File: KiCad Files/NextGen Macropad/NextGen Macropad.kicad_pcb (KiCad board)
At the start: 2 copper layers, 80.4 x 119.4 mm, 80 parts, among them J1 OLED_128x64, J2 Battery JST-PH, J3 USB_C_Receptacle_USB2.0_16P, Q1 AO3401A, SW1 SW_Push_45deg, SW10 SW_Push_45deg, SW11 SW_Push_45deg, SW12 SW_Push_45deg, SW13 SW_Push_45deg, SW14 SW_Push_45deg, SW15 SW_Push_45deg, SW16 SW_Push_45deg, SW17 SW_DP3T, SW18 Reset, SW19 Boot, SW2 SW_Push_45deg, SW3 SW_Push_45deg, SW4 SW_Push_45deg, SW5 SW_Push_45deg, SW6 SW_Push_45deg, SW7 SW_Push_45deg, SW8 SW_Push_45deg, SW9 SW_Push_45deg, U1 ESP32-S3-WROOM-1, U2 TP4056-42-ESOP8, U3 AP2112K-3.3

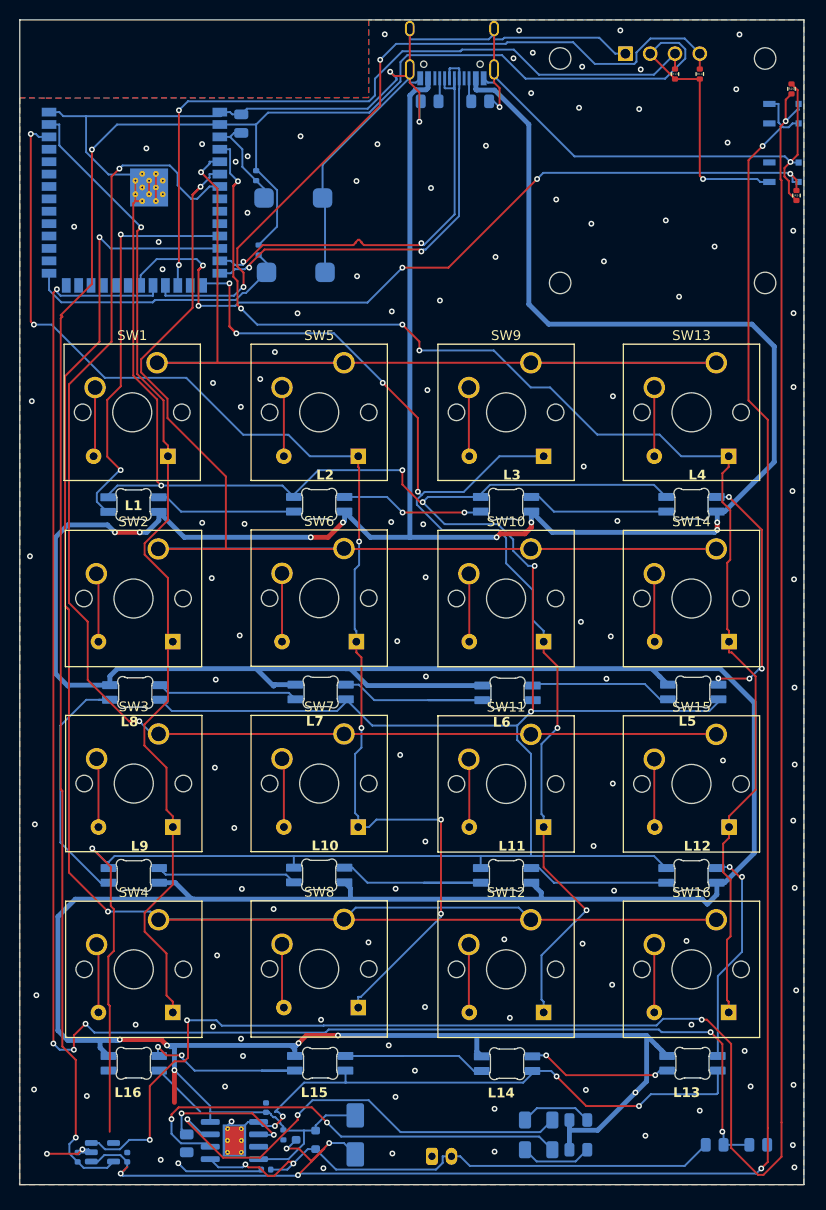
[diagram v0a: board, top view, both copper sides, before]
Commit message: New PCB Layout
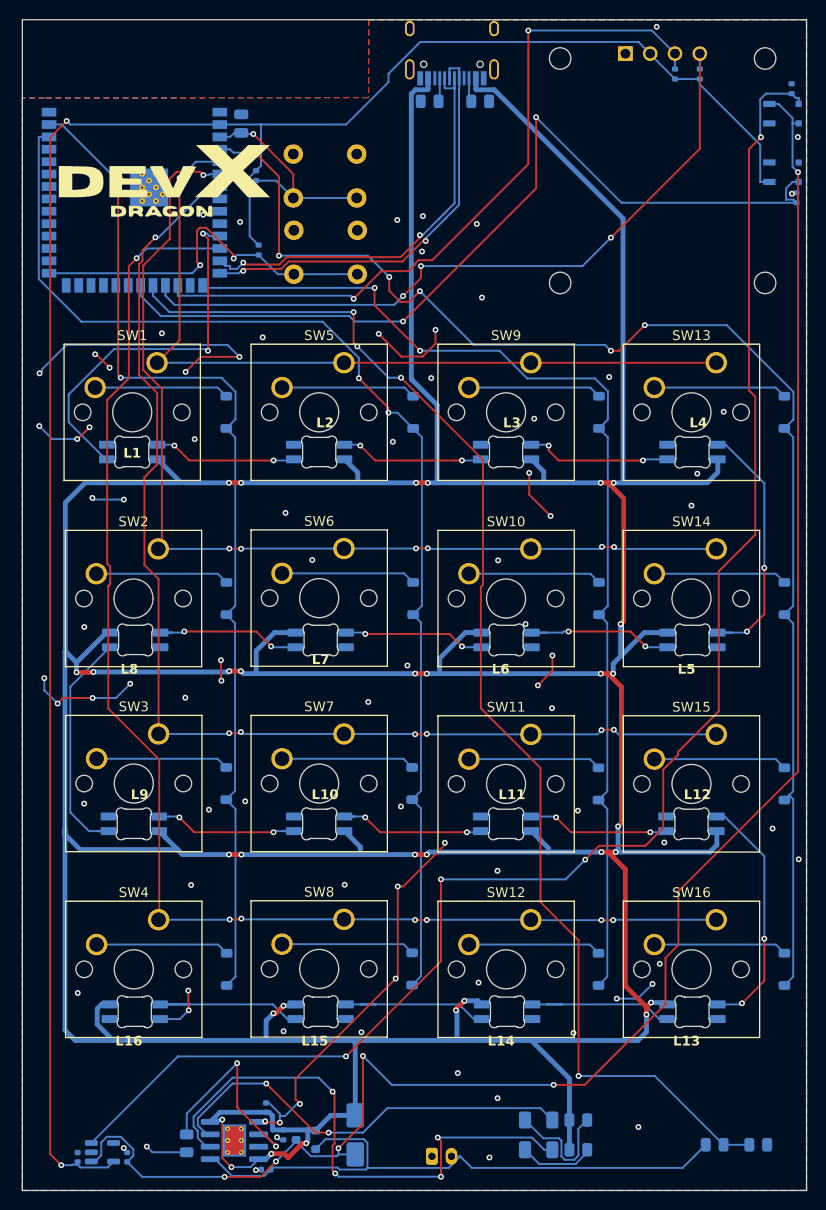
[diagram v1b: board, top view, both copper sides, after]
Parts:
- added G***: LOGO, Dragon Emblem:White DevX Official Logo, F.Cu at (89.8, 60.4)
- added G***: LOGO, Dragon Emblem:White DevX Official Logo, B.Cu at (141.7, 58.7)
- D1, D10, D11, D12, D13, D14, D15, D16, D2, D3, D4, D5, D6, D7, D8, D9: footprint ScottoKeebs_Components:Diode_DO-35 -> ScottoKeebs_Components:Diode_SOD-123
- R10, R13, R14, R9: moved to B.Cu
- SW18, SW19: footprint Button_Switch_SMD:SW_Push_1TS009xxxx-xxxx-xxxx_6x6x5mm -> Button_Switch_THT:SW_PUSH_6mm
- moved D1 7.48 mm to (97.0, 83.5), turned to 90 degrees
- moved D6 7.30 mm to (116.2, 102.5), turned to 90 degrees
- moved D13 7.27 mm to (154.2, 83.5), turned to 90 degrees
- moved D9 7.24 mm to (135.2, 83.5), turned to 90 degrees
- moved D16 7.22 mm to (154.2, 140.5), turned to 90 degrees
- moved D5 7.20 mm to (116.2, 83.5), turned to 90 degrees
- moved D10 7.19 mm to (135.2, 102.5), turned to 90 degrees
- moved D14 7.19 mm to (154.2, 102.5), turned to 90 degrees
- moved D15 7.19 mm to (154.2, 121.5), turned to 90 degrees
- moved D12 7.15 mm to (135.2, 140.5), turned to 90 degrees
- moved D11 7.15 mm to (135.2, 121.5), turned to 90 degrees
- moved D7 7.10 mm to (116.1, 121.5), turned to 90 degrees
- moved D4 7.08 mm to (97.1, 140.5), turned to 90 degrees
- moved D3 7.06 mm to (97.0, 121.5), turned to 90 degrees
- moved D2 7.05 mm to (97.0, 102.5), turned to 90 degrees
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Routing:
- net GND: track 565.3 -> 129.4 mm, vias 134 -> 86
- net /COLO 3: track 187.3 -> 137.7 mm, vias 2 -> 7
- net /REG - EN: track 208.1 -> 161.4 mm
- net /VOLT-DIV: track 173.7 -> 131.5 mm, vias 6 -> 4
- net /COLO 1: track 143.5 -> 103.0 mm, vias 1 -> 7
- net /COLO 2: track 157.7 -> 120.0 mm, vias 2 -> 7
- net /COLO 0: track 118.2 -> 82.0 mm
- net +5V: track 551.0 -> 583.8 mm, vias 14 -> 32
- net /MOSFET: track 202.1 -> 181.6 mm
- net /RESET PIN: track 10.1 -> 22.9 mm, vias 0 -> 1
- net /ROW 2: track 121.9 -> 110.6 mm, vias 6 -> 2
- net /Boot: track 28.1 -> 38.5 mm, vias 0 -> 2
- net /ROW 1: track 131.1 -> 121.1 mm, vias 6 -> 2
- net +3.3V: track 221.9 -> 212.1 mm, vias 3 -> 2
- net Net-(U2-~{STDBY}): track 47.6 -> 56.6 mm, vias 2 -> 4
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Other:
- board size 80.4 x 119.4 mm -> 80.4 x 120 mm
- board text added: "+"
- board text added: "-"
